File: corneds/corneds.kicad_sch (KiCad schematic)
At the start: 130 parts, among them J1 Conn_ARM_SWD_TagConnect_TC203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, J2 Conn_ARM_SWD_TagConnect_TC203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, J3 AudioJack4, J4 AudioJack4, SW1 SW_Push, SW10 SW_Push, SW11 SW_Push, SW12 SW_Push, SW13 SW_Push, SW14 SW_Push, SW15 SW_Push, SW16 SW_Push, SW17 SW_Push, SW18 SW_Push, SW19 SW_Push, SW2 SW_Push, SW20 SW_Push, SW21 SW_Push, SW22 SW_Push, SW23 SW_Push, SW24 SW_Push, SW25 SW_Push, SW26 SW_Push, SW27 SW_Push, SW28 SW_Push, SW29 SW_Push, SW3 SW_Push, SW30 SW_Push, SW31 SW_Push, SW32 SW_Push, SW33 SW_Push, SW34 SW_Push, SW35 SW_Push, SW36 SW_Push, SW37 SW_Push, SW38 SW_Push, SW39 SW_Push, SW4 SW_Push, SW40 SW_Push, SW41 SW_Push, SW42 SW_Push, SW5 SW_Push, SW6 SW_Push, SW7 SW_Push, SW8 SW_Push, SW9 SW_Push, U1 Pico, U2 Pico

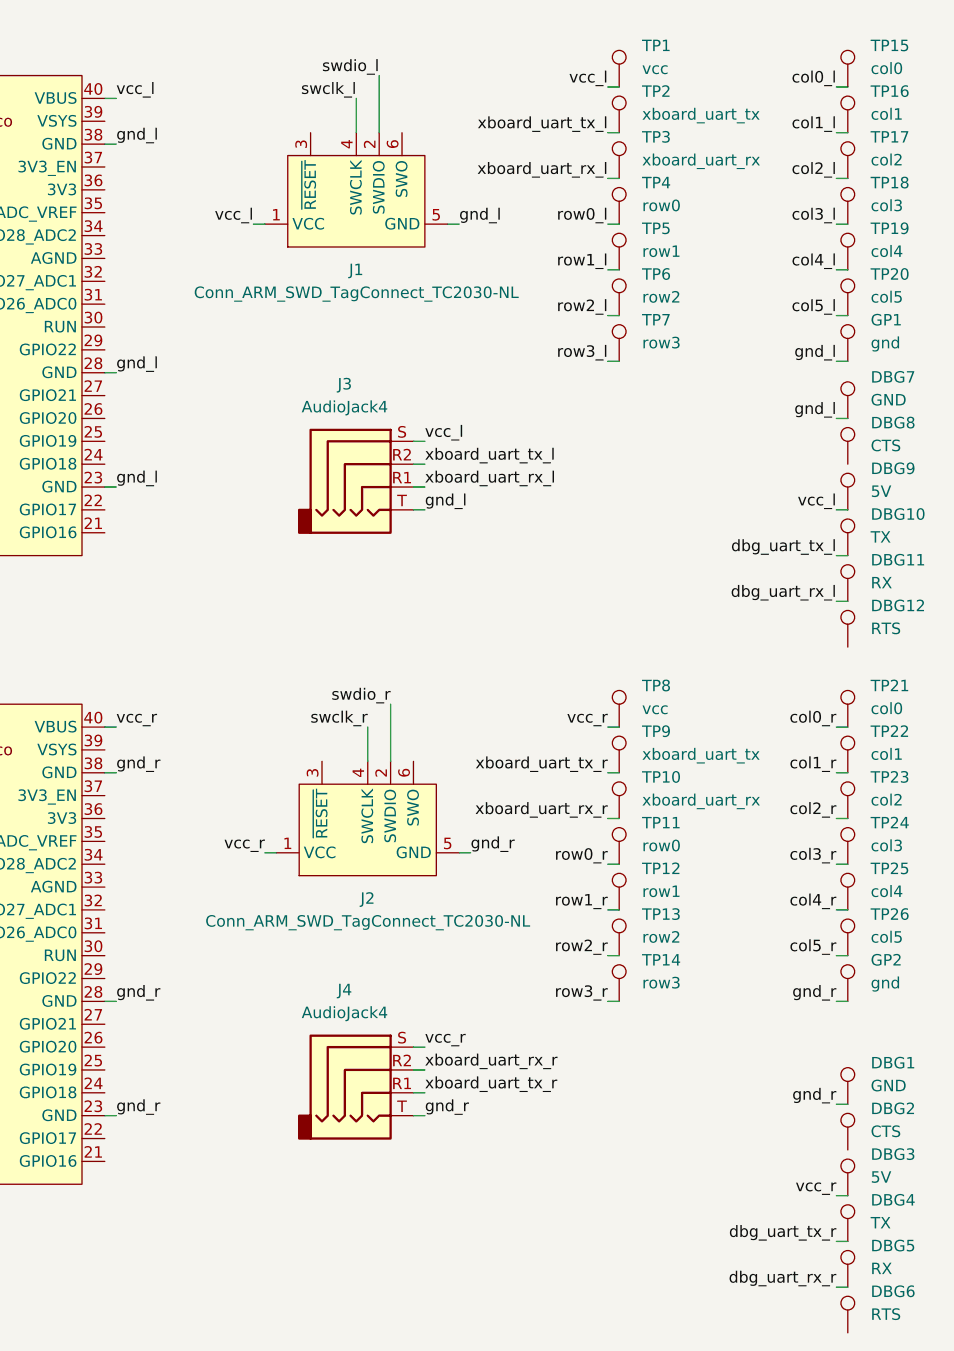
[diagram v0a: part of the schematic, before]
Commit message: ordered version
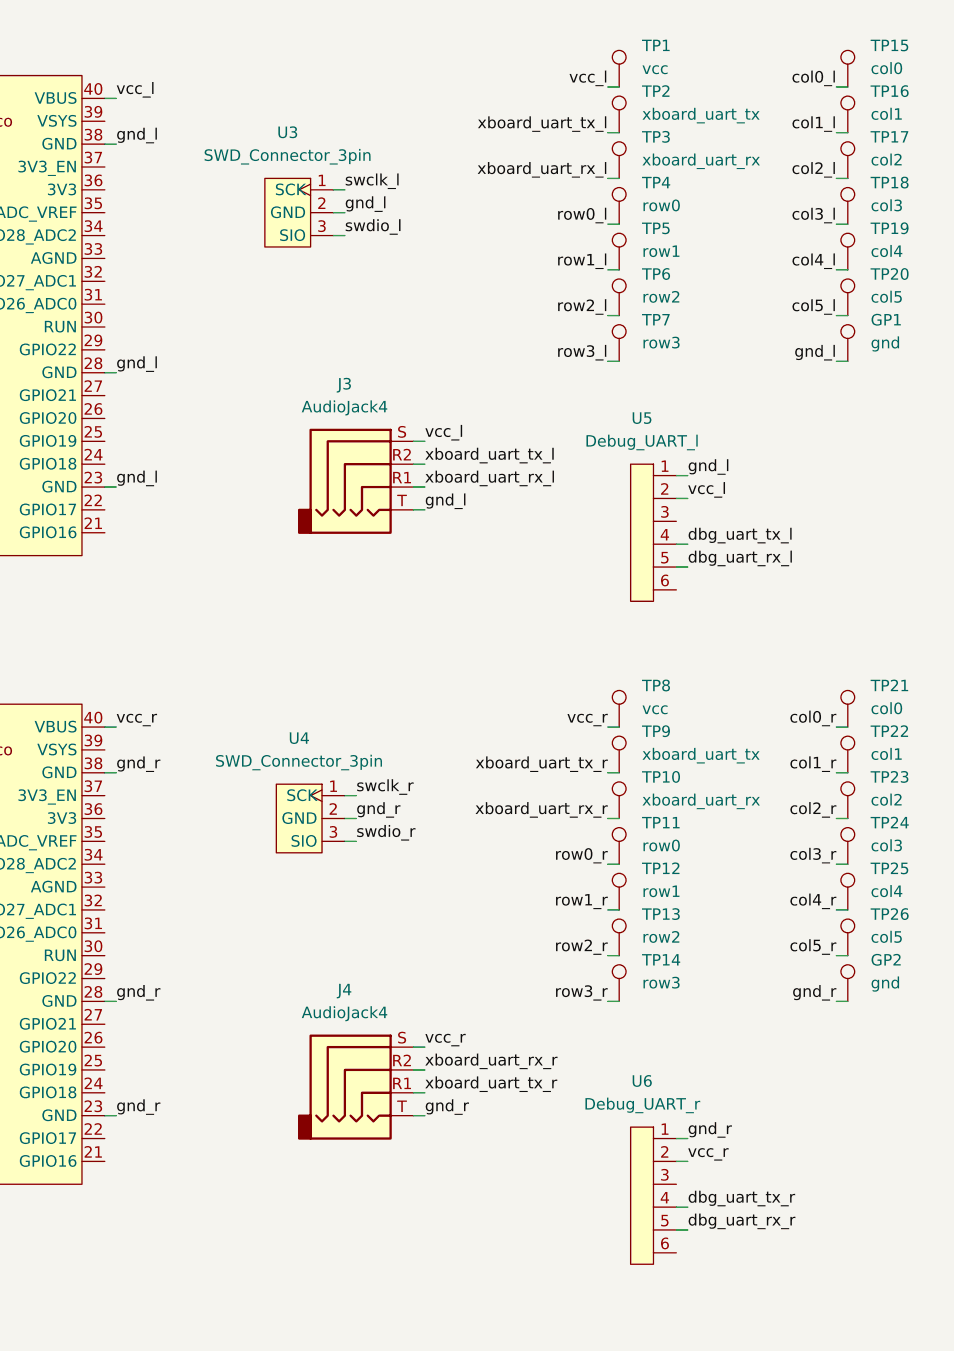
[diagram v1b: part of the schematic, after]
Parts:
- removed DBG1, DBG7: GND, Connector_PinSocket_2.54mm:PinSocket_1x01_P2.54mm_Vertical, symbol Connector:TestPoint
- removed DBG10, DBG4: TX, Connector_PinSocket_2.54mm:PinSocket_1x01_P2.54mm_Vertical, symbol Connector:TestPoint
- removed DBG11, DBG5: RX, Connector_PinSocket_2.54mm:PinSocket_1x01_P2.54mm_Vertical, symbol Connector:TestPoint
- removed DBG12, DBG6: RTS, Connector_PinSocket_2.54mm:PinSocket_1x01_P2.54mm_Vertical, symbol Connector:TestPoint
- removed DBG2, DBG8: CTS, Connector_PinSocket_2.54mm:PinSocket_1x01_P2.54mm_Vertical, symbol Connector:TestPoint
- removed DBG3, DBG9: 5V, Connector_PinSocket_2.54mm:PinSocket_1x01_P2.54mm_Vertical, symbol Connector:TestPoint
- removed J1, J2: Conn_ARM_SWD_TagConnect_TC2030-NL, Connector:Tag-Connect_TC2030-IDC-NL_2x03_P1.27mm_Vertical, symbol Connector:Conn_ARM_SWD_TagConnect_TC2030-NL
- added U3, U4: SWD_Connector_3pin, entropy:SM03B-SRSS-TB, symbol entropy:SWD_Connector_3pin
- added U5: Debug_UART_l, entropy:Header_6pin, symbol entropy:Header_6pin
- added U6: Debug_UART_r, entropy:Header_6pin, symbol entropy:Header_6pin
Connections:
- net dbg_uart_rx_l: now also U5.5
- net dbg_uart_rx_r: now also U6.5
- net dbg_uart_tx_l: now also U5.4
- net dbg_uart_tx_r: now also U6.4
- net gnd_l: now also U3.2 (GND), U5.1
- net gnd_r: now also U4.2 (GND), U6.1
- net swclk_l: now also U3.1 (SCK)
- net swclk_r: now also U4.1 (SCK)
- net swdio_l: now also U3.3 (SIO)
- net swdio_r: now also U4.3 (SIO)
- net vcc_l: now also U5.2
- net vcc_r: now also U6.2
